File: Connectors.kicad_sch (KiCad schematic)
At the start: 4 parts, among them J1 Conn_01x09, J2 Conn_01x04, J3 Conn_02x03_Odd_Even, J4 Conn_01x04

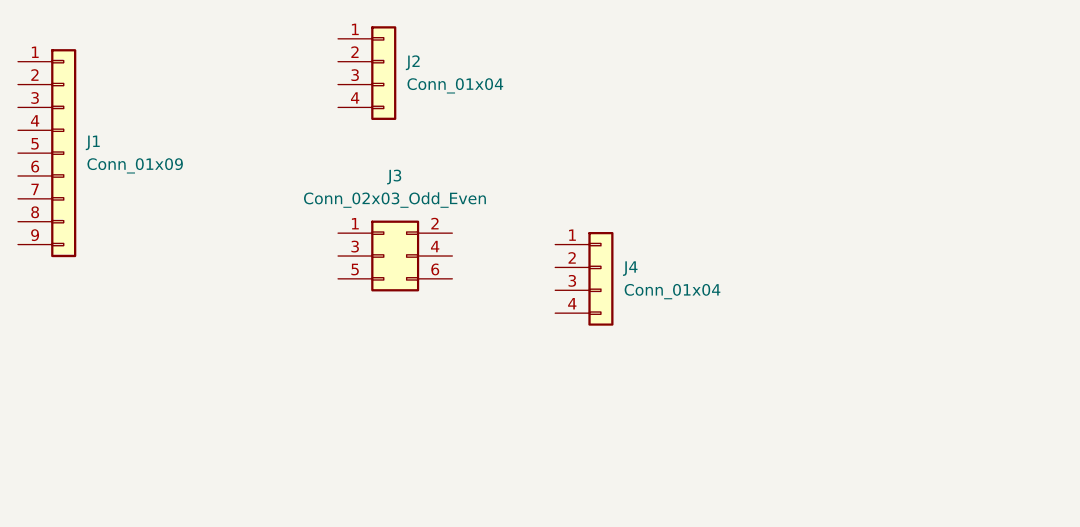
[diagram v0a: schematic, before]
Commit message: Arranged symbols
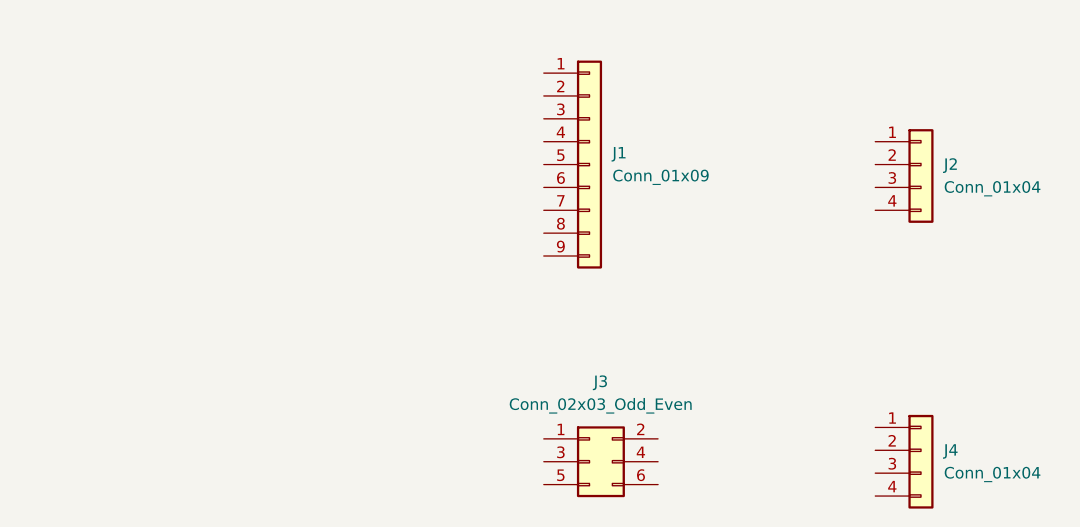
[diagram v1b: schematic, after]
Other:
- moved on the sheet: J1, J2, J3, J4
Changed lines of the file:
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@@
 	(symbol
 		(lib_id "Connector_Generic:Conn_02x03_Odd_Even")
-		(at 97.79 90.17 0)
+		(at 120.65 113.03 0)
 		(unit 1)
 		(exclude_from_sim no)
@@
 		(fields_autoplaced yes)
 		(property "Reference" "J3"
-			(at 99.06 81.28 0)
+			(at 121.92 104.14 0)
 			(effects
 				(font
@@
 		)
 		(property "Value" "Conn_02x03_Odd_Even"
-			(at 99.06 83.82 0)
-			(effects
-				(font
-					(size 1.27 1.27)
-				)
-			)
-		)
-		(property "Footprint" ""
-			(at 97.79 90.17 0)
-			(effects
-				(font
-					(size 1.27 1.27)
-				)
-				(hide yes)
-			)
-		)
-		(property "Datasheet" "~"
-			(at 97.79 90.17 0)
+			(at 121.92 106.68 0)
+			(effects
+				(font
+					(size 1.27 1.27)
+				)
+			)
+		)
+		(property "Footprint" ""
+			(at 120.65 113.03 0)
+			(effects
+				(font
+					(size 1.27 1.27)
+				)
+				(hide yes)
+			)
+		)
+		(property "Datasheet" "~"
+			(at 120.65 113.03 0)
 			(effects
 				(font
@@
 		)
 		(property "Description" "Generic connector, double row, 02x03, odd/even pin numbering scheme (row 1 odd numbers, row 2 even numbers), script generated (kicad-library-utils/schlib/autogen/connector/)"
-			(at 97.79 90.17 0)
+			(at 120.65 113.03 0)
 			(effects
 				(font
@@
 	(symbol
 		(lib_id "Connector_Generic:Conn_01x04")
-		(at 97.79 68.58 0)
+		(at 157.48 80.01 0)
 		(unit 1)
 		(exclude_from_sim no)
@@
 		(fields_autoplaced yes)
 		(property "Reference" "J2"
-			(at 100.33 68.5799 0)
+			(at 160.02 80.0099 0)
 			(effects
 				(font
@@
 		)
 		(property "Value" "Conn_01x04"
-			(at 100.33 71.1199 0)
-			(effects
-				(font
-					(size 1.27 1.27)
-				)
-				(justify left)
-			)
-		)
-		(property "Footprint" ""
-			(at 97.79 68.58 0)
-			(effects
-				(font
-					(size 1.27 1.27)
-				)
-				(hide yes)
-			)
-		)
-		(property "Datasheet" "~"
-			(at 97.79 68.58 0)
+			(at 160.02 82.5499 0)
+			(effects
+				(font
+					(size 1.27 1.27)
+				)
+				(justify left)
+			)
+		)
+		(property "Footprint" ""
+			(at 157.48 80.01 0)
+			(effects
+				(font
+					(size 1.27 1.27)
+				)
+				(hide yes)
+			)
+		)
+		(property "Datasheet" "~"
+			(at 157.48 80.01 0)
 			(effects
 				(font
@@
 		)
 		(property "Description" "Generic connector, single row, 01x04, script generated (kicad-library-utils/schlib/autogen/connector/)"
-			(at 97.79 68.58 0)
+			(at 157.48 80.01 0)
 			(effects
 				(font
@@
 	(symbol
 		(lib_id "Connector_Generic:Conn_01x09")
-		(at 62.23 78.74 0)
+		(at 120.65 80.01 0)
 		(unit 1)
 		(exclude_from_sim no)
@@
 		(fields_autoplaced yes)
 		(property "Reference" "J1"
-			(at 64.77 77.4699 0)
+			(at 123.19 78.7399 0)
 			(effects
 				(font
@@
 		)
 		(property "Value" "Conn_01x09"
-			(at 64.77 80.0099 0)
-			(effects
-				(font
-					(size 1.27 1.27)
-				)
-				(justify left)
-			)
-		)
-		(property "Footprint" ""
-			(at 62.23 78.74 0)
-			(effects
-				(font
-					(size 1.27 1.27)
-				)
-				(hide yes)
-			)
-		)
-		(property "Datasheet" "~"
-			(at 62.23 78.74 0)
+			(at 123.19 81.2799 0)
+			(effects
+				(font
+					(size 1.27 1.27)
+				)
+				(justify left)
+			)
+		)
+		(property "Footprint" ""
+			(at 120.65 80.01 0)
+			(effects
+				(font
+					(size 1.27 1.27)
+				)
+				(hide yes)
+			)
+		)
+		(property "Datasheet" "~"
+			(at 120.65 80.01 0)
 			(effects
 				(font
@@
 		)
 		(property "Description" "Generic connector, single row, 01x09, script generated (kicad-library-utils/schlib/autogen/connector/)"
-			(at 62.23 78.74 0)
+			(at 120.65 80.01 0)
 			(effects
 				(font
@@
 	(symbol
 		(lib_id "Connector_Generic:Conn_01x04")
-		(at 121.92 91.44 0)
+		(at 157.48 111.76 0)
 		(unit 1)
 		(exclude_from_sim no)
@@
 		(fields_autoplaced yes)
 		(property "Reference" "J4"
-			(at 124.46 91.4399 0)
+			(at 160.02 111.7599 0)
 			(effects
 				(font
@@
 		)
 		(property "Value" "Conn_01x04"
-			(at 124.46 93.9799 0)
-			(effects
-				(font
-					(size 1.27 1.27)
-				)
-				(justify left)
-			)
-		)
-		(property "Footprint" ""
-			(at 121.92 91.44 0)
-			(effects
-				(font
-					(size 1.27 1.27)
-				)
-				(hide yes)
-			)
-		)
-		(property "Datasheet" "~"
-			(at 121.92 91.44 0)
+			(at 160.02 114.2999 0)
+			(effects
+				(font
+					(size 1.27 1.27)
+				)
+				(justify left)
+			)
+		)
+		(property "Footprint" ""
+			(at 157.48 111.76 0)
+			(effects
+				(font
+					(size 1.27 1.27)
+				)
+				(hide yes)
+			)
+		)
+		(property "Datasheet" "~"
+			(at 157.48 111.76 0)
 			(effects
 				(font
@@
 		)
 		(property "Description" "Generic connector, single row, 01x04, script generated (kicad-library-utils/schlib/autogen/connector/)"
-			(at 121.92 91.44 0)
-			(effects
-				(font
+			(at 157.48 111.76 0)
+			(effects
+				(font
